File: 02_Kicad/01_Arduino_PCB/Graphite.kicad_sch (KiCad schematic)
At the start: 17 parts, among them J1 Power, J2 Digital/PWM, J3 Analog, J4 Digital/PWM, U1 LTC1050, U2 HC05

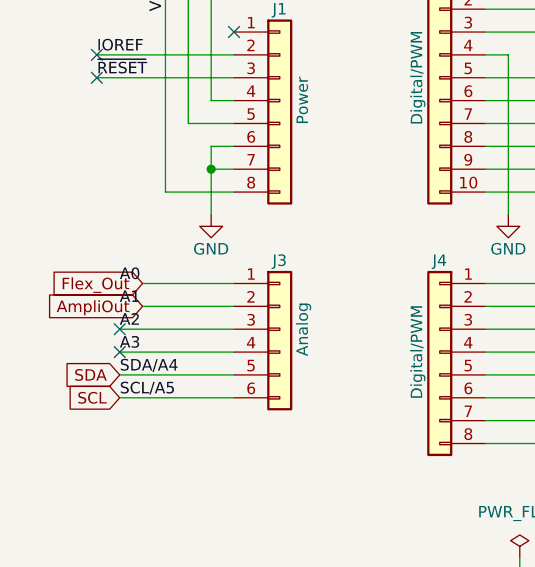
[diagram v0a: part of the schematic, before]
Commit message: Ajout Nouvelles mesures
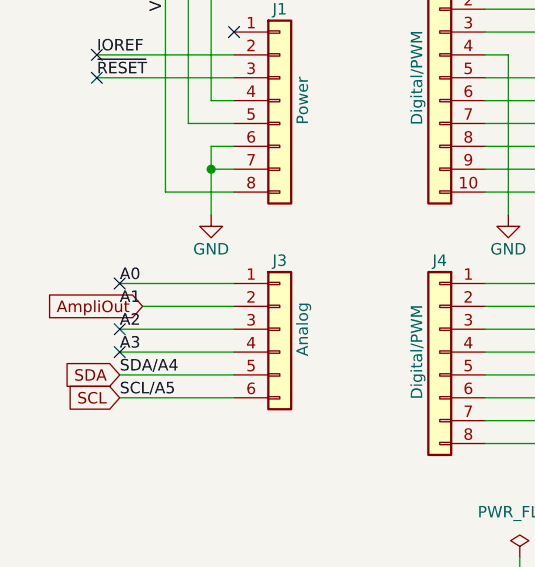
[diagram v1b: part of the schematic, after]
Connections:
- net A0: now also J3.1 (Pin_1)
- net Flex_Out: no longer J3.1 (Pin_1)
- no-connect marks 22 -> 23
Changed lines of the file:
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@@
+	)
+	(no_connect
+		(at 21.59 59.69)
 	)
 	(no_connect
@@
 	(wire
 		(pts
-			(xy 24.13 59.69) (xy 34.29 59.69)
-		)
-		(stroke
-			(width 0)
-			(type default)
-		)
-	)
-	(wire
-		(pts
 			(xy 215.9 133.35) (xy 215.9 139.7)
 		)
@@
 		(pts
 			(xy 87.63 134.62) (xy 91.44 134.62)
+		)
+		(stroke
+			(width 0)
+			(type default)
+		)
+	)
+	(wire
+		(pts
+			(xy 21.59 59.69) (xy 34.29 59.69)
 		)
 		(stroke
@@
 			(effects
 				(font
-					(size 1.27 1.27)
-				)
-				(justify right)
-				(hide yes)
-			)
-		)
-	)
-	(global_label "Flex_Out"
-		(shape input)
-		(at 24.13 59.69 180)
-		(fields_autoplaced yes)
-		(effects
-			(font
-				(size 1.27 1.27)
-			)
-			(justify right)
-		)
-		(property "Intersheetrefs" "${INTERSHEET_REFS}"
-			(at 13.0064 59.69 0)
-			(effects
-				(font
